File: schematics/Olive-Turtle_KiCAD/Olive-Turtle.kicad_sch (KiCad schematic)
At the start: 4 parts, among them IC1 ENS160-BGLT, U1 ESP32-DEVKITC-32U

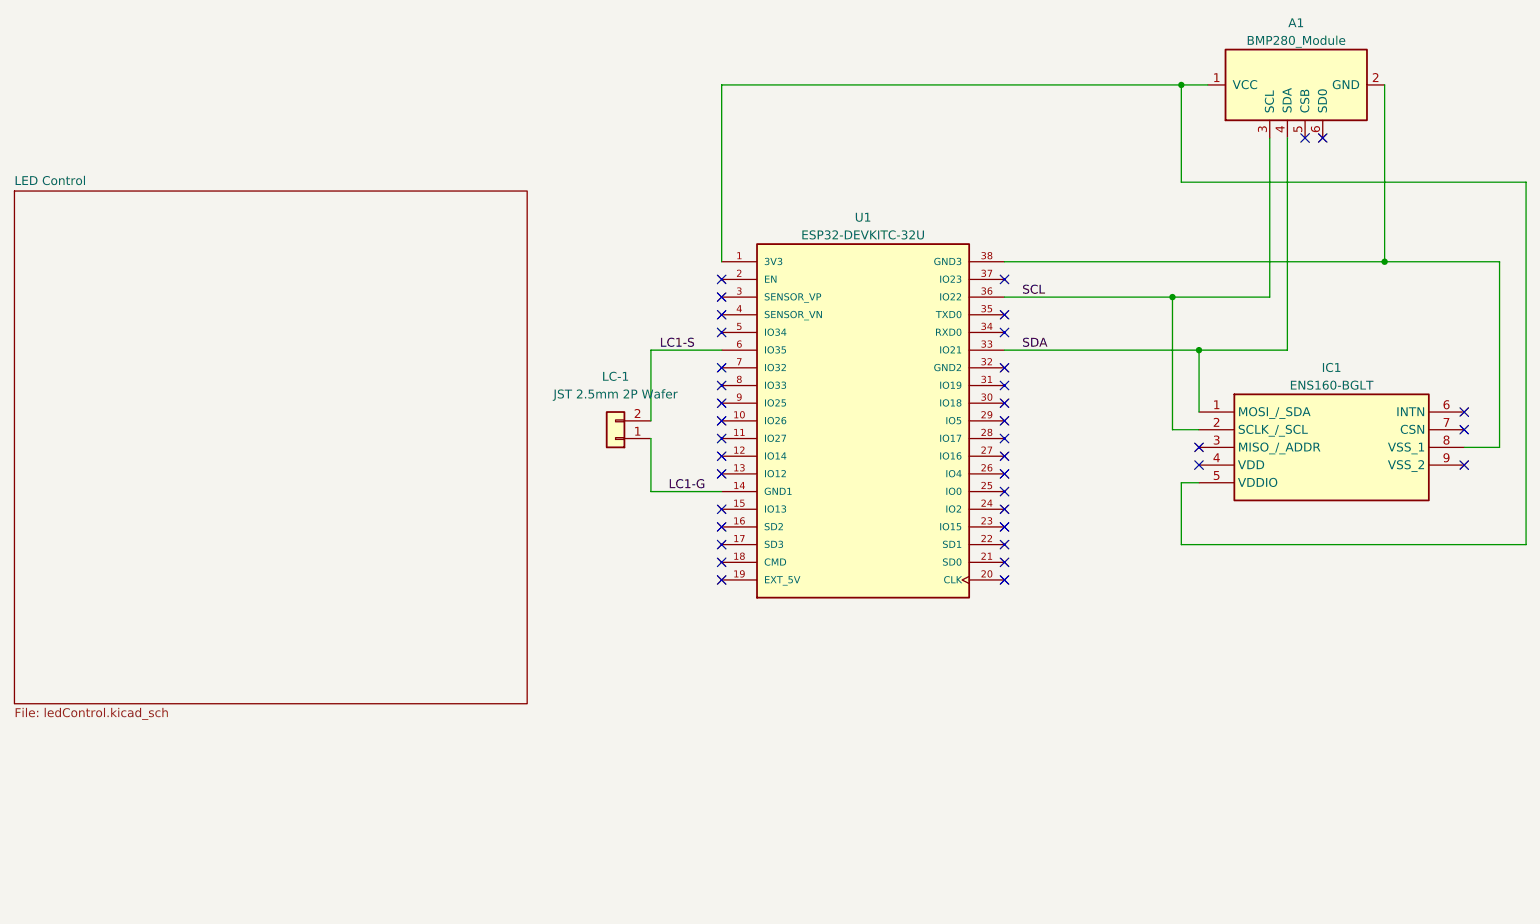
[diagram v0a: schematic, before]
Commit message: [develop] Update Kicad schematic
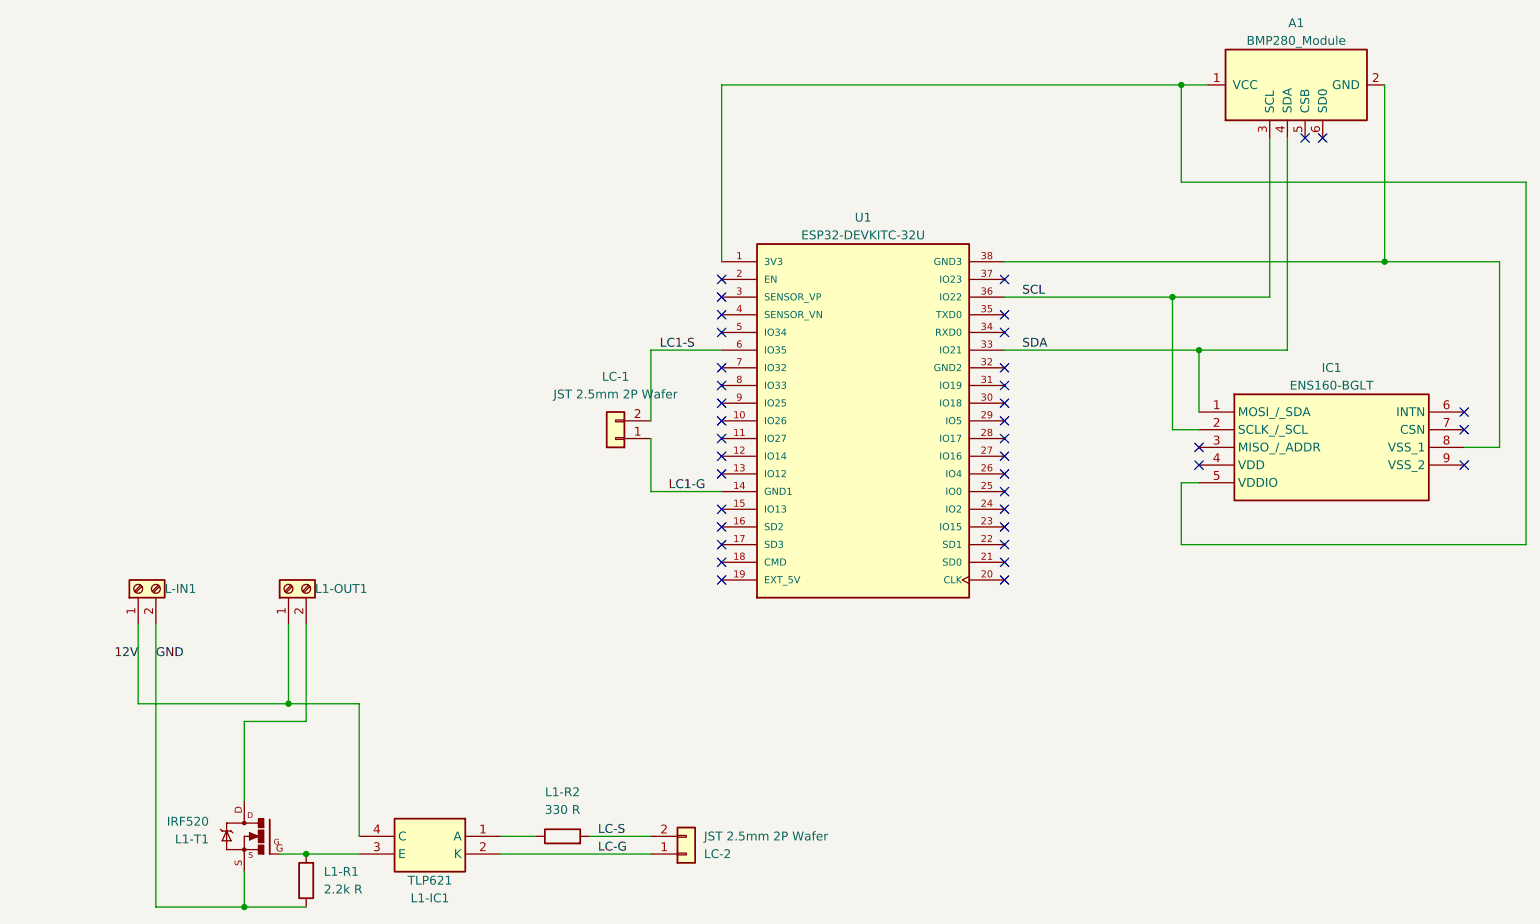
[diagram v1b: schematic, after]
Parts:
- added L-IN1, L1-OUT1: Screw_Terminal_01x02, TerminalBlock:TerminalBlock_bornier-2_P5.08mm, symbol Connector:Screw_Terminal_01x02
- added L1-IC1: TLP621, DIP762W60P254L460H450Q4N, symbol TLP621:TLP621
- added L1-R1: 2.2k R, Resistor_THT:R_Axial_DIN0204_L3.6mm_D1.6mm_P7.62mm_Horizontal, symbol Device:R
- added L1-R2: 330 R, Resistor_THT:R_Axial_DIN0204_L3.6mm_D1.6mm_P7.62mm_Horizontal, symbol Device:R
- added L1-T1: IRF520, TO220BV, symbol IRF520:IRF520
- added LC-2: JST 2.5mm 2P Wafer, Connector_JST:JST_EH_B2B-EH-A_1x02_P2.50mm_Vertical, symbol Connector_Generic:Conn_01x02
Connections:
- new net: L1-OUT1.2 (Pin_2), L1-T1.D
- new net: L1-IC1.3 (E), L1-R1.2, L1-T1.G
- new net: L1-IC1.1 (A), L1-R2.1
- new net 12V: L-IN1.1 (Pin_1), L1-IC1.4 (C), L1-OUT1.1 (Pin_1)
- new net GND: L-IN1.2 (Pin_2), L1-R1.1, L1-T1.S
- new net LC-G: L1-IC1.2 (K), LC-2.1 (Pin_1)
- new net LC-S: L1-R2.2, LC-2.2 (Pin_2)
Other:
- removed sheet LED Control
